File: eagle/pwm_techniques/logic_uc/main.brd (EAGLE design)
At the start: 74 x 58.7 mm, 32 parts, among them IC1 LM2936MP-3.0, IC2 317EMP, U1 SN74LS08D, U2 SN74HCT04D, U3 ARDUINOR3-DIMENSION

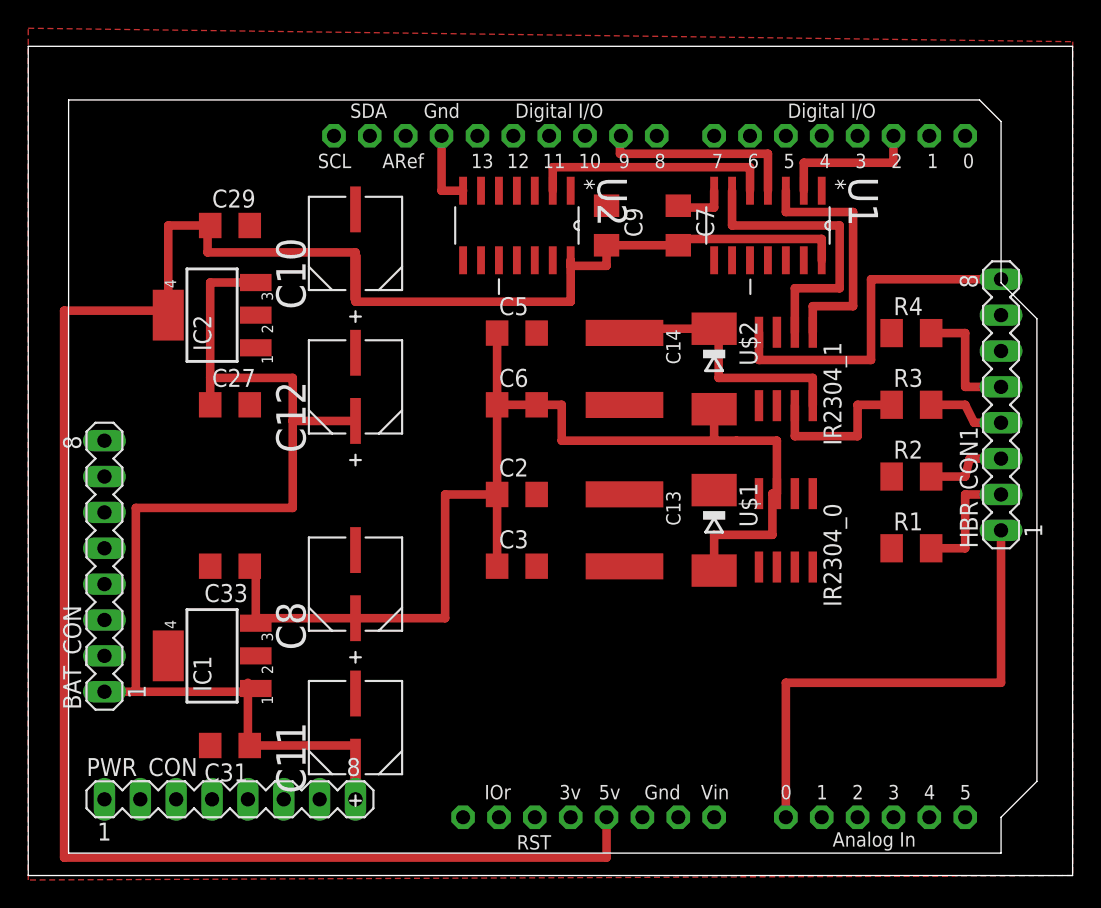
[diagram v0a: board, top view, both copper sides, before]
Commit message: [ update ] logic_uc board routed
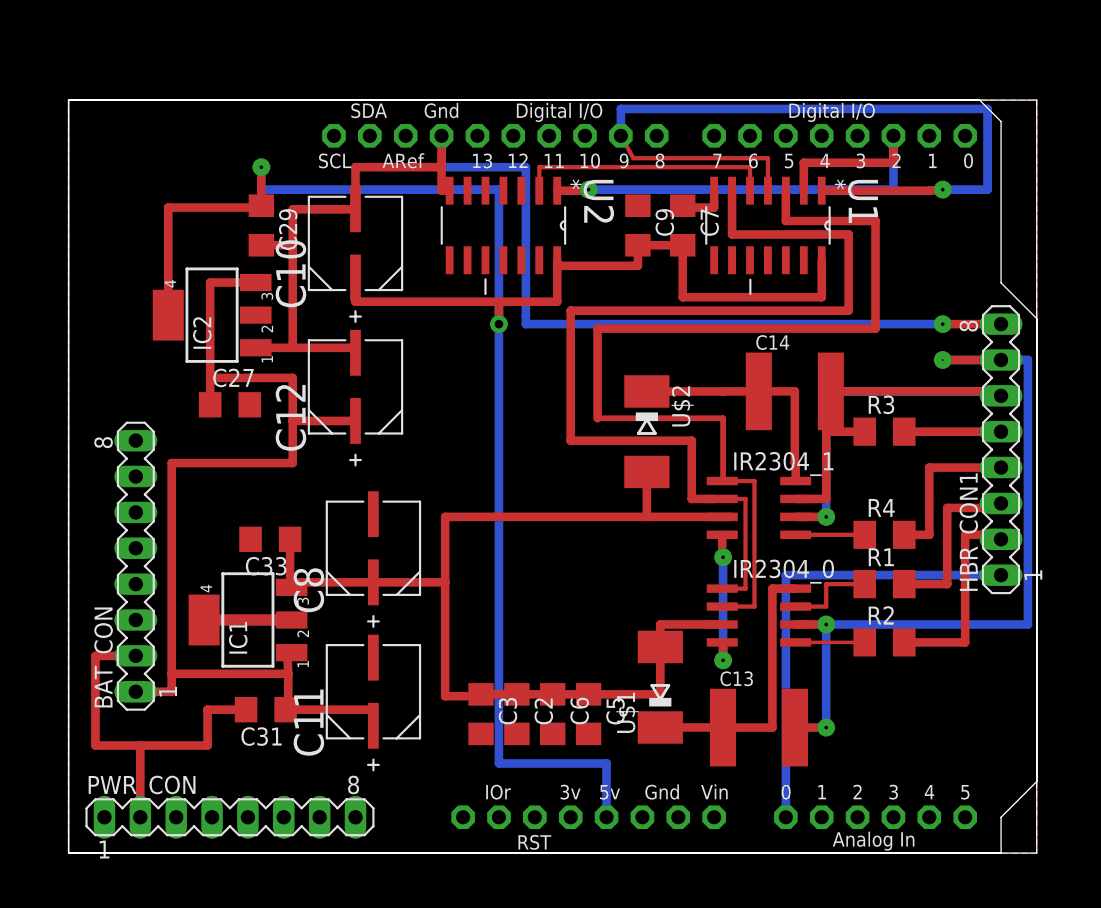
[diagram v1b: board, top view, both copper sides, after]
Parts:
- moved C5 27.5 mm to (36.8, 9.84), turned to 270 degrees
- moved C6 22.1 mm to (34.3, 9.84), turned to 270 degrees
- moved C13 16.9 mm to (48.9, 8.89), turned to 0 degrees
- moved C2 15.6 mm to (31.8, 9.84), turned to 270 degrees
- moved R4 14.4 mm to (57.8, 22.5)
- moved C14 12.2 mm to (51.4, 32.7), turned to 0 degrees
- moved R2 11.9 mm to (57.8, 14.9)
- moved U$1 11.7 mm to (41.9, 11.7), turned to 90 degrees
- moved C3 10.8 mm to (29.2, 9.84), turned to 270 degrees
- moved IR2304_1 10.0 mm to (48.9, 24.4), turned to 270 degrees
- moved U$2 6.51 mm to (41.0, 29.8)
- moved IR2304_0 6.33 mm to (48.9, 16.8), turned to 270 degrees
- moved C31 3.59 mm to (14.0, 10.2)
- moved IC1 3.59 mm to (12.7, 16.5)
- moved C33 3.43 mm to (14.3, 22.2)
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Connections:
- net Q0_GATE: now also HBR_CON1.3; no longer HBR_CON1.2
- net Q1_GATE: now also HBR_CON1.2; no longer HBR_CON1.3
- net Q2_GATE: now also HBR_CON1.5; no longer HBR_CON1.4
- net Q3_GATE: now also HBR_CON1.4; no longer HBR_CON1.5
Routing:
- net GND: track 34.1 -> 132.2 mm, vias 0 -> 3
- net LOAD_P: track 0.00 -> 54.9 mm, vias 0 -> 3
- net CTL_SIDE_0: track 17.6 -> 68.9 mm
- net CTL_SIDE_1: track 20.8 -> 69.6 mm
- net CTL_PWM: track 14.4 -> 59.0 mm, vias 0 -> 1
- net LOAD_N: track 0.00 -> 36.1 mm, vias 0 -> 1
- net CTL_DIR: track 10.2 -> 37.9 mm, vias 0 -> 1
- net N$1: track 0.00 -> 19.4 mm
- net VREG_5: track 152.5 -> 134.6 mm, vias 0 -> 3
- net VREG_10: track 85.4 -> 75.4 mm
- net Q1_GATE: track 5.94 -> 14.8 mm
- net N$3: track 0.00 -> 6.48 mm
- net N$8: track 0.00 -> 6.20 mm
- net N$7: track 0.00 -> 4.89 mm
- net N$4: track 0.00 -> 4.89 mm
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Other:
- board size 74 x 58.7 mm -> 68.6 x 53.3 mm
